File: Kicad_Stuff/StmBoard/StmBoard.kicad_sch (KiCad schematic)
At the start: 46 parts, among them J1 USB_B_Mini, SW1 SW_DIP_x01, SW2 SW_DIP_x01, SW3 SW_DIP_x01, SW4 SW_DIP_x01, SW5 SW_DIP_x01, SW6 SW_DIP_x01, SW7 SW_DIP_x01, SW8 SW_DIP_x01, SW9 SW_DIP_x01, U1 STM32G031K8Tx, U13 MCP2221AxST, U2 LIS3DH, U8 MIC5504-3.3YM5, U9 L78L05_SO8, Y1 32Khz LSE

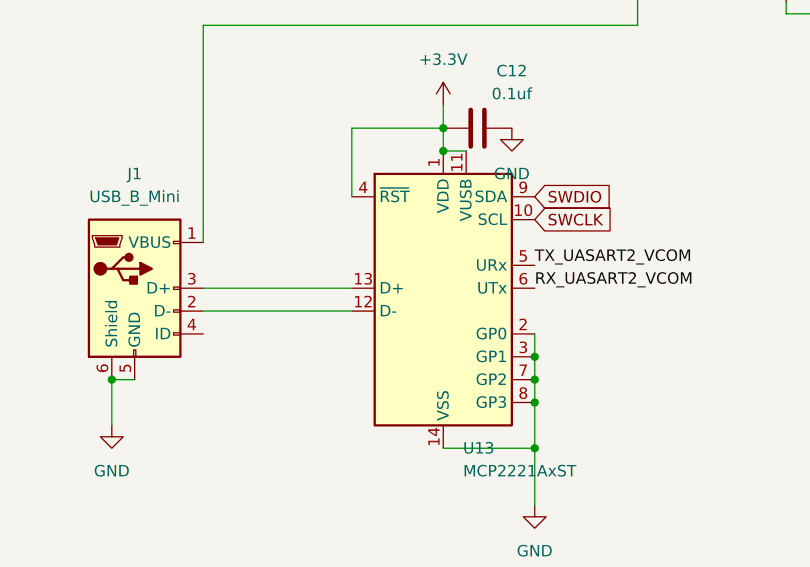
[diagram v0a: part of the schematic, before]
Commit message: quick commit
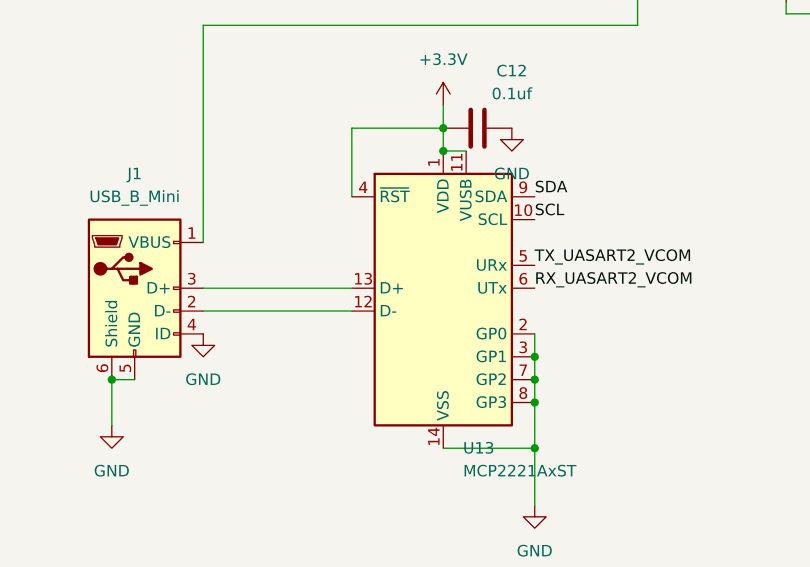
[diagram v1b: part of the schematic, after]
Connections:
- net GND: now also J1.4 (ID)
- net SCL: now also U13.10 (SCL)
- net SDA: now also U13.9 (SDA)
- net SWCLK: no longer U13.10 (SCL)
- net SWDIO: no longer U13.9 (SDA)
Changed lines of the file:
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@@
+    (effects (font (size 1.27 1.27)) (justify left bottom))
+  )
+  (label "SDA" (at 162.56 149.86 0) (fields_autoplaced)
+    (effects (font (size 1.27 1.27)) (justify left bottom))
+  )
+  (label "SCL" (at 162.56 152.4 0) (fields_autoplaced)
     (effects (font (size 1.27 1.27)) (justify left bottom))
   )
@@
     )
   )
-  (global_label "SWCLK" (shape input) (at 162.56 152.4 0) (fields_autoplaced)
-    (effects (font (size 1.27 1.27)) (justify left))
-    (property "Intersheetrefs" "${INTERSHEET_REFS}" (at 171.7742 152.4 0)
-      (effects (font (size 1.27 1.27)) (justify left) hide)
-    )
-  )
-  (global_label "SWDIO" (shape input) (at 162.56 149.86 0) (fields_autoplaced)
-    (effects (font (size 1.27 1.27)) (justify left))
-    (property "Intersheetrefs" "${INTERSHEET_REFS}" (at 171.4114 149.86 0)
-      (effects (font (size 1.27 1.27)) (justify left) hide)
-    )
-  )
   (symbol (lib_id "Switch:SW_DIP_x01") (at 26.67 125.73 0) (unit 1)
     (in_bom yes) (on_board yes) (dnp no) (fields_autoplaced)
@@
         )
       )
+    )
+  )
+  (symbol (lib_id "power:GND") (at 125.73 165.1 0) (unit 1)
+    (in_bom yes) (on_board yes) (dnp no) (fields_autoplaced)
+    (property "Reference" "#PWR039" (at 125.73 171.45 0)
+      (effects (font (size 1.27 1.27)) hide)
+    )
+    (property "Value" "GND" (at 125.73 170.18 0)
+      (effects (font (size 1.27 1.27)))
+    )
+    (property "Footprint" "" (at 125.73 165.1 0)
+      (effects (font (size 1.27 1.27)) hide)
+    )
+    (property "Datasheet" "" (at 125.73 165.1 0)
+      (effects (font (size 1.27 1.27)) hide)
+    )
+    (pin "1")
+    (instances
+      (project "StmBoard"
+        (path "/27842249-4d05-45e0-a285-5f644f3ee952"
+          (reference "#PWR039") (unit 1)
+        )
+      )
